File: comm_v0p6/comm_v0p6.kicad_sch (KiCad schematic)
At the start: 12 parts, among them J1 1x15 header, J2 1x15 socket, J4 2x2 socket, J5 2x2 socket, J6 2x2 socket, J7 2x2 socket, U1 ATmega328PB-M, Y1 20MHz

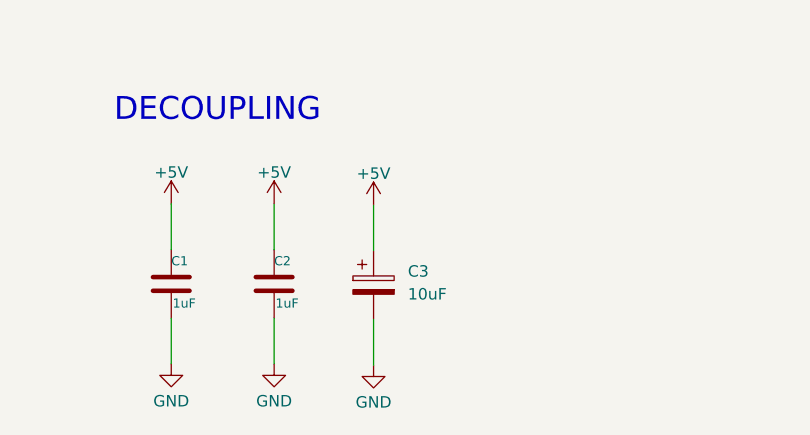
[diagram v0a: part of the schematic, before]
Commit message: Made BOM and CPL files for comm_v0p6 design.  Need to test.
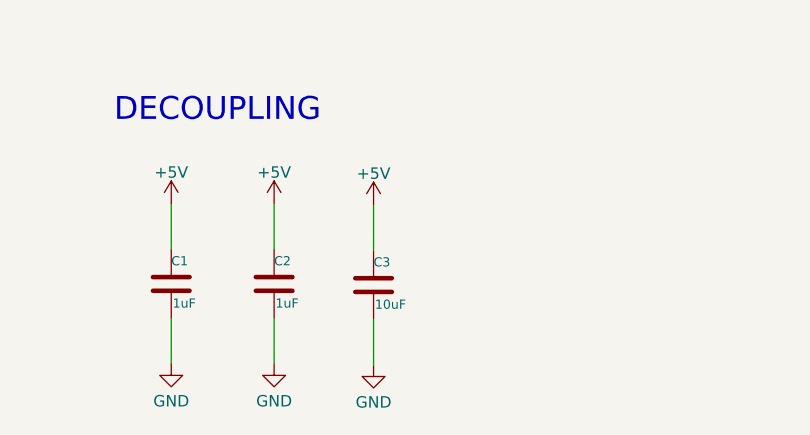
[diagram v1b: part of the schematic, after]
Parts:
- removed C3: 10uF, Capacitor_SMD:C_0805_2012Metric, symbol Device:C_Polarized
- added C3: 10uF, Capacitor_SMD:C_0805_2012Metric, symbol Device:C
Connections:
- net +5V: now also C3.1
- net GND: now also C3.2
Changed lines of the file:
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@@
+    )
+  )
+  (symbol (lib_id "Device:C") (at 65.786 168.529 0) (unit 1)
+    (in_bom yes) (on_board yes) (dnp no)
+    (property "Reference" "C3" (at 65.786 165.989 0)
+      (effects (font (size 1.016 1.016)) (justify left))
+    )
+    (property "Value" "10uF" (at 65.9384 170.688 0)
+      (effects (font (size 1.016 1.016)) (justify left))
+    )
+    (property "Footprint" "Capacitor_SMD:C_0805_2012Metric" (at 66.7512 172.339 0)
+      (effects (font (size 0.762 0.762)) hide)
+    )
+    (property "Datasheet" "https://media.digikey.com/pdf/Data%20Sheets/Samsung%20PDFs/CL10B104KO8NNNC_Spec.pdf" (at 65.786 168.529 0)
+      (effects (font (size 1.524 1.524)) hide)
+    )
+    (property "PN" "CL10B104KO8NNNC" (at 65.786 168.529 0)
+      (effects (font (size 1.27 1.27)) hide)
+    )
+    (property "DigiKey PN" "1276-1067-1-ND" (at 65.786 168.529 0)
+      (effects (font (size 1.27 1.27)) hide)
+    )
+    (property "LCSC PN" "C5137499" (at 65.786 168.529 0)
+      (effects (font (size 1.27 1.27)) hide)
+    )
+    (pin "1")
+    (pin "2")
+    (instances
+      (project "comm_v0p6"
+        (path "/4a438c85-e5df-473f-b41d-177df9356b07"
+          (reference "C3") (unit 1)
+        )
+      )
     )
   )
@@
         )
       )
-    )
-  )
-  (symbol (lib_id "Device:C_Polarized") (at 65.786 168.529 0) (unit 1)
-    (in_bom yes) (on_board yes) (dnp no) (fields_autoplaced)
-    (property "Reference" "C3" (at 69.596 167.005 0)
-      (effects (font (size 1.27 1.27)) (justify left))
-    )
-    (property "Value" "10uF" (at 69.596 169.545 0)
-      (effects (font (size 1.27 1.27)) (justify left))
-    )
-    (property "Footprint" "Capacitor_SMD:C_0805_2012Metric" (at 66.7512 172.339 0)
-      (effects (font (size 1.27 1.27)) hide)
-    )
-    (property "Datasheet" "~" (at 65.786 168.529 0)
-      (effects (font (size 1.27 1.27)) hide)
-    )
-    (property "LCSC PN" "C72484" (at 65.786 168.529 0)
-      (effects (font (size 1.27 1.27)) hide)
-    )
-    (pin "1")
-    (pin "2")
-    (instances
-      (project "comm_v0p6"
-        (path "/4a438c85-e5df-473f-b41d-177df9356b07"
-          (reference "C3") (unit 1)
-        )
-      )
